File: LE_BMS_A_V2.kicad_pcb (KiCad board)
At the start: 4 copper layers, 80 x 80 mm, 57 parts, among them J1 10155435-00011LF, J2 CAN1, J3 691382010012, J4 691313510002, J5 RJHSE5380, J6 CAN1, U1 ESP32-S3-WROOM-2, U2 MCP2515-xST, U3 ISO1050DUB, U4 ISO1050DUB, U5 TLV1117LV33DCYT, U6 DS3231MZ, Y1 ABM3B-8.000MHZ-10-1-U-T

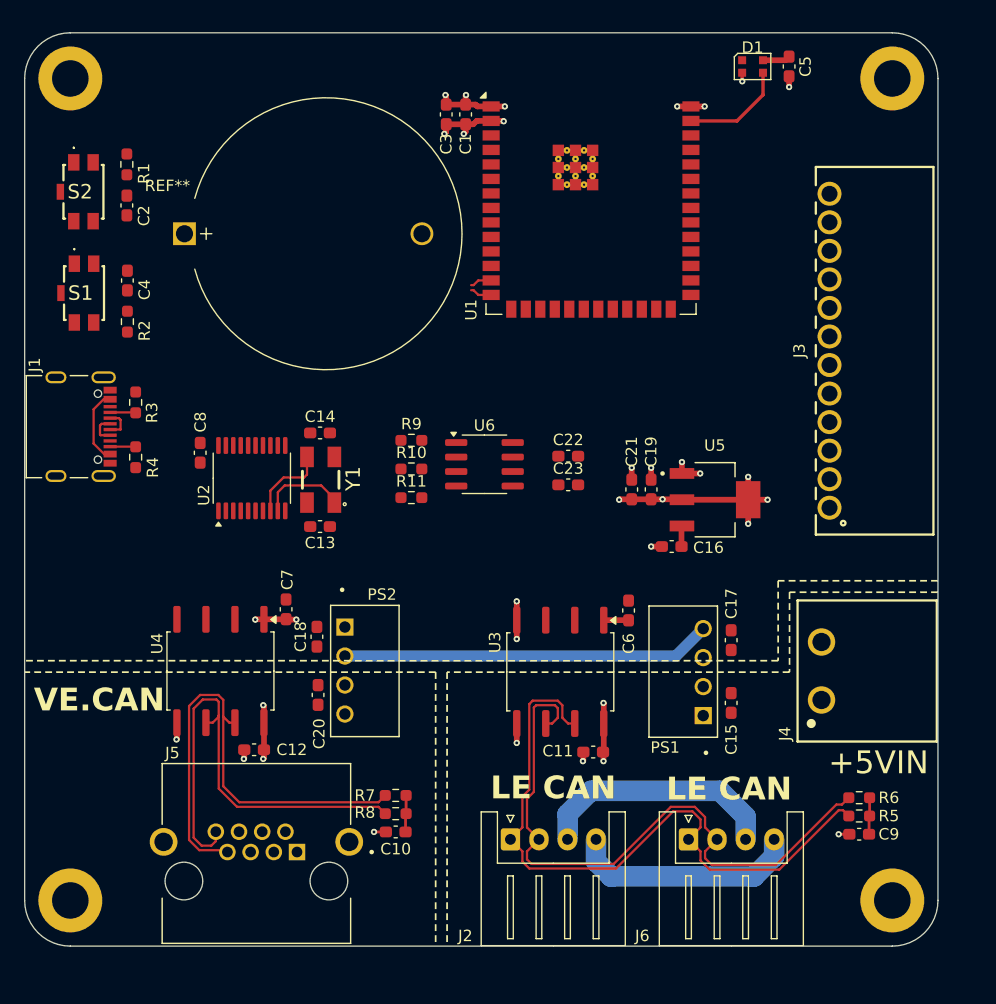
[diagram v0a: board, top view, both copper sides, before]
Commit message: Finished most routing, final checks to be done
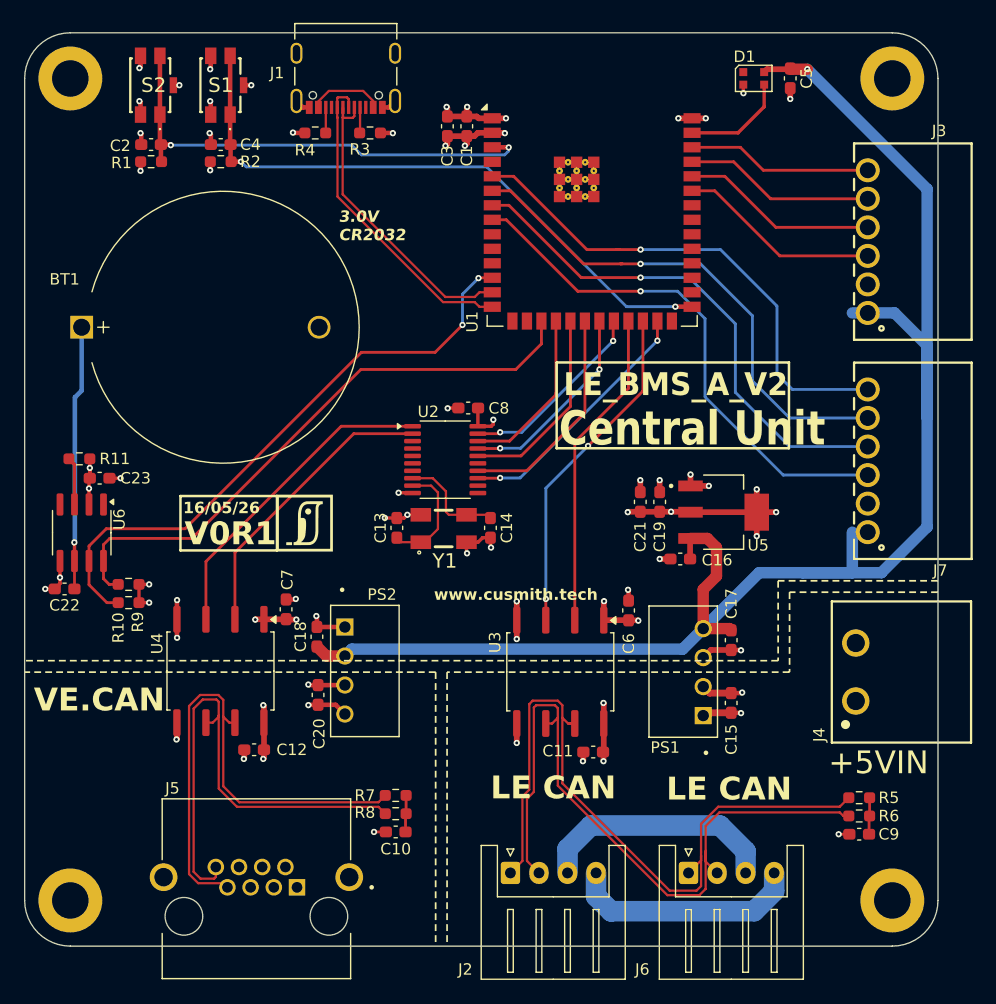
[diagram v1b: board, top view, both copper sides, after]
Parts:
- removed REF**: BatteryHolder_MYOUNG_BS-07-A1BJ001_CR2032, Battery:BatteryHolder_MYOUNG_BS-07-A1BJ001_CR2032
- added BT1: Battery_Cell, Battery:BatteryHolder_MYOUNG_BS-07-A1BJ001_CR2032, F.Cu at (118.1, 72.4)
- added G***: LOGO, LOGO, F.Cu at (137.7, 89.5)
- added J7: 691382010006, 691382010006:691382010006, F.Cu at (187.0, 84.1)
- J3: value 691382010012 -> 691382010006; footprint 691382010012:691382010012 -> 691382010006:691382010006
- moved C22 45.6 mm to (116.6, 95.3), turned to 180 degrees
- moved J1 41.4 mm to (141.3, 48.4), turned to 180 degrees
- moved C23 41.0 mm to (119.7, 85.6)
- moved U6 35.8 mm to (118.2, 90.4), turned to -90 degrees
- moved R4 32.5 mm to (138.6, 55.4), turned to 180 degrees
- moved R3 31.3 mm to (143.4, 55.4), turned to 180 degrees
- moved R11 29.3 mm to (117.9, 83.9), turned to 180 degrees
- moved R9 27.8 mm to (122.3, 94.9)
- moved R10 27.4 mm to (122.3, 96.5), turned to 180 degrees
- moved C8 23.8 mm to (152.0, 79.5), turned to 180 degrees
- moved S1 21.8 mm to (130.3, 51.2), turned to 180 degrees
- moved C14 17.1 mm to (153.9, 90.0), turned to -90 degrees
- moved U2 17.0 mm to (150.0, 84.0), turned to 0 degrees
- moved R2 16.2 mm to (130.3, 57.9), turned to 0 degrees
- moved C4 14.4 mm to (130.3, 56.4), turned to 180 degrees
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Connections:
- J3 pad 1: unconnected-(J3-Pad1) -> +5V
- J3 pad 2: unconnected-(J3-Pad2) -> GND
- J3 pad 3: unconnected-(J3-Pad3) -> /Project Architecture/Section A - Title A/GPIO_A1
- J3 pad 4: unconnected-(J3-Pad4) -> /Project Architecture/Section A - Title A/GPIO_A2
- J3 pad 5: unconnected-(J3-Pad5) -> /Project Architecture/Section A - Title A/GPIO_A3
- J3 pad 6: unconnected-(J3-Pad6) -> /Project Architecture/Section A - Title A/GPIO_A4
- R10 pad 2: /Project Architecture/Section A - Title A/SDA -> /Project Architecture/Section A - Title A/I2C_SDA
- R9 pad 1: /Project Architecture/Section A - Title A/SCL -> /Project Architecture/Section A - Title A/I2C_SCL
- U1 pad 12: unconnected-(U1-IO8-Pad12) -> /Project Architecture/Section A - Title A/I2C_SDA
- U1 pad 17: /Project Architecture/Section A - Title A/CAN2_INT -> /Project Architecture/Section A - Title A/I2C_SCL
- U1 pad 25: unconnected-(U1-IO48-Pad25) -> /Project Architecture/Section A - Title A/CAN2_INT
- U1 pad 35: unconnected-(U1-MTMS/IO42-Pad35) -> /Project Architecture/Section A - Title A/GPIO_A1
- U1 pad 36: unconnected-(U1-RXD0/IO44-Pad36) -> /Project Architecture/Section A - Title A/GPIO_A2
- U1 pad 37: unconnected-(U1-TXD0/IO43-Pad37) -> /Project Architecture/Section A - Title A/GPIO_A3
- U1 pad 38: unconnected-(U1-IO2-Pad38) -> /Project Architecture/Section A - Title A/GPIO_A4
- U1 pad 5: unconnected-(U1-IO5-Pad5) -> /Project Architecture/Section A - Title A/GPIO_B4
- U1 pad 6: unconnected-(U1-IO6-Pad6) -> /Project Architecture/Section A - Title A/GPIO_B3
- U1 pad 7: unconnected-(U1-IO7-Pad7) -> /Project Architecture/Section A - Title A/GPIO_B2
- U1 pad 8: unconnected-(U1-IO15-Pad8) -> /Project Architecture/Section A - Title A/GPIO_B1
- U6 pad 7: /Project Architecture/Section A - Title A/SDA -> /Project Architecture/Section A - Title A/I2C_SDA
- U6 pad 8: /Project Architecture/Section A - Title A/SCL -> /Project Architecture/Section A - Title A/I2C_SCL
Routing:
- net +5V: track 36.6 -> 143.3 mm, vias 0 -> 1
- net /Project Architecture/Section A - Title A/ESP32_BOOT: track 0.00 -> 54.9 mm, vias 0 -> 2
- net /Project Architecture/Section A - Title A/I2C_SDA: track 0.00 -> 53.2 mm, vias 0 -> 2
- net /Project Architecture/Section A - Title A/I2C_SCL: track 0.00 -> 52.1 mm
- net /Project Architecture/Section A - Title A/GPIO_B1: track 0.00 -> 46.2 mm, vias 0 -> 1
- net /Project Architecture/Section A - Title A/GPIO_B2: track 0.00 -> 45.2 mm, vias 0 -> 1
- net /Project Architecture/Section A - Title A/GPIO_B3: track 0.00 -> 44.6 mm, vias 0 -> 1
- net /Project Architecture/Section A - Title A/GPIO_B4: track 0.00 -> 44.4 mm, vias 0 -> 1
- net /Project Architecture/Section A - Title A/ESP32_EN: track 0.00 -> 42.1 mm, vias 0 -> 2
- net GND: track 19.9 -> 59.0 mm, vias 14 -> 39
- net /Project Architecture/Section A - Title A/CAN1_TX: track 0.00 -> 29.7 mm, vias 0 -> 2
- net /Project Architecture/Section A - Title A/CAN1_RX: track 0.00 -> 28.1 mm
- net /Project Architecture/Section B - Title B/CAN2_TX: track 0.00 -> 28.1 mm
- net /Project Architecture/Section B - Title B/CAN2_RX: track 0.00 -> 25.7 mm
- net /Project Architecture/Section A - Title A/ESP32_USB_D+: track 5.03 -> 28.5 mm
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- added copper zone on In2.Cu, net +5V_CAN2
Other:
- board text added: "16/05/26"
- board text added: "3.0V CR2032"
- board text added: "Central Unit"
- board text added: "LE_BMS_A_V2"
- board text added: "V0R1"
- board text added: "www.cusmith.tech"
